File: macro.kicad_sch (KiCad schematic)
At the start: 50 parts, among them J1 Conn_01x01_Male, J2 Conn_01x01_Male, J3 Conn_01x01_Male, SW1 RotaryEncoder_Switch, SW2 SW_Push, U1 AP2112K-3.3, U2 W25Q128JVPIQ, U3 RP2040, Y1 12MHz

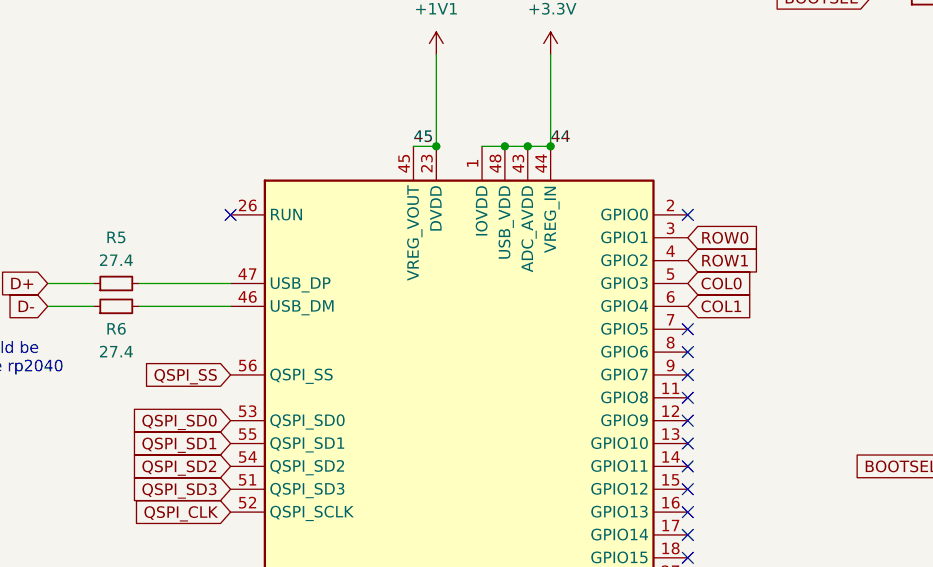
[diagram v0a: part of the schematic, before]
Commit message: v0
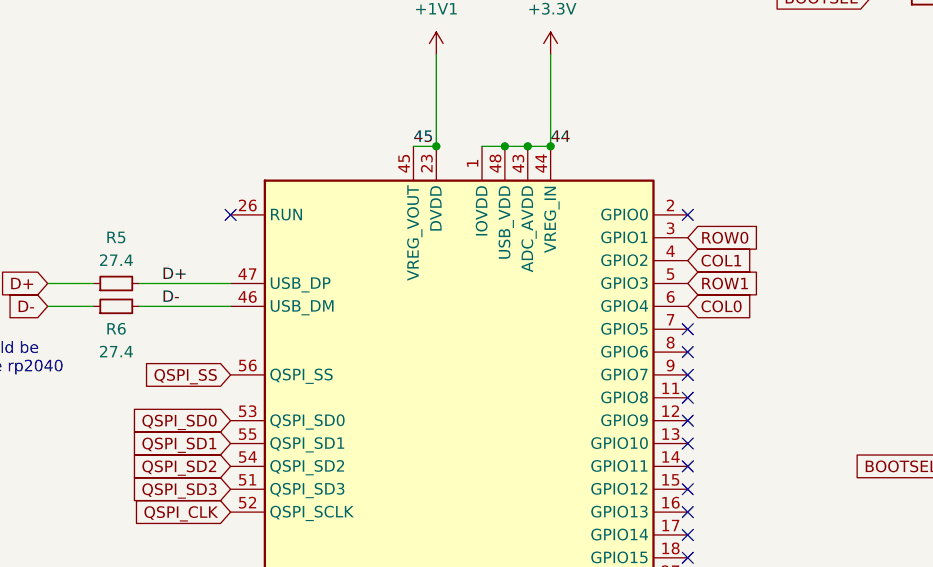
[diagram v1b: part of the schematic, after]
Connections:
- net COL0: now also U3.6 (GPIO4); no longer U3.5 (GPIO3)
- net COL1: now also U3.4 (GPIO2); no longer U3.6 (GPIO4)
- net D+: now also R5.2, U3.47 (USB_DP)
- net D-: now also R6.2, U3.46 (USB_DM)
- net ROW1: now also U3.5 (GPIO3); no longer U3.4 (GPIO2)
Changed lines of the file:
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@@
+    (effects (font (size 1.27 1.27)) (justify left bottom))
+  )
+  (label "D-" (at 41.91 115.57 0)
     (effects (font (size 1.27 1.27)) (justify left bottom))
   )
   (label "44" (at 128.27 184.15 0)
+    (effects (font (size 1.27 1.27)) (justify left bottom))
+  )
+  (label "D+" (at 41.91 113.03 0)
     (effects (font (size 1.27 1.27)) (justify left bottom))
   )
@@
     )
   )
-  (global_label "ROW1" (shape input) (at 100.33 110.49 0) (fields_autoplaced)
+  (global_label "ROW1" (shape input) (at 100.33 113.03 0) (fields_autoplaced)
     (effects (font (size 1.27 1.27)) (justify left))
-    (property "Intersheet References" "${INTERSHEET_REFS}" (id 0) (at 108.0045 110.4106 0)
+    (property "Intersheet References" "${INTERSHEET_REFS}" (id 0) (at 108.0045 112.9506 0)
       (effects (font (size 1.27 1.27)) (justify left) hide)
     )
@@
     )
   )
-  (global_label "COL1" (shape input) (at 100.33 115.57 0) (fields_autoplaced)
+  (global_label "COL1" (shape input) (at 100.33 110.49 0) (fields_autoplaced)
     (effects (font (size 1.27 1.27)) (justify left))
-    (property "Intersheet References" "${INTERSHEET_REFS}" (id 0) (at 107.5812 115.4906 0)
+    (property "Intersheet References" "${INTERSHEET_REFS}" (id 0) (at 107.5812 110.4106 0)
       (effects (font (size 1.27 1.27)) (justify left) hide)
     )
@@
     )
   )
-  (global_label "COL0" (shape input) (at 100.33 113.03 0) (fields_autoplaced)
+  (global_label "COL0" (shape input) (at 100.33 115.57 0) (fields_autoplaced)
     (effects (font (size 1.27 1.27)) (justify left))
-    (property "Intersheet References" "${INTERSHEET_REFS}" (id 0) (at 107.5812 112.9506 0)
+    (property "Intersheet References" "${INTERSHEET_REFS}" (id 0) (at 107.5812 115.4906 0)
       (effects (font (size 1.27 1.27)) (justify left) hide)
     )
